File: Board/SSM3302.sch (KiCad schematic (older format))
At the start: 5 parts, among them U2 SSM3302ACPZ-R7

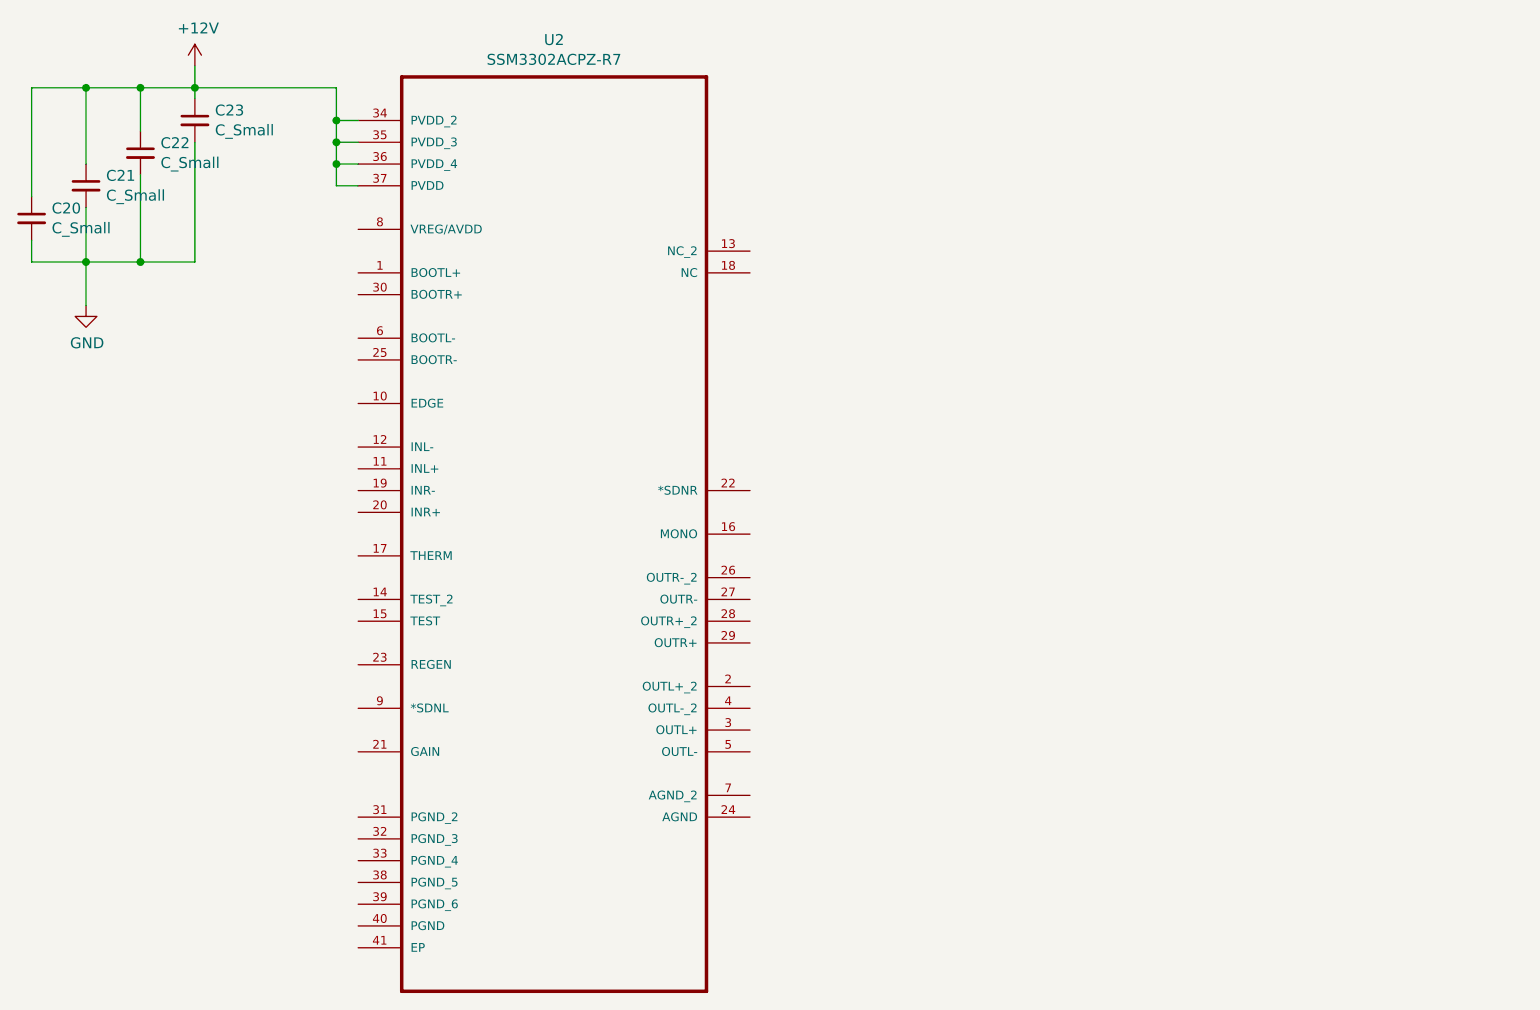
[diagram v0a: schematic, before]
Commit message: did some more stuff
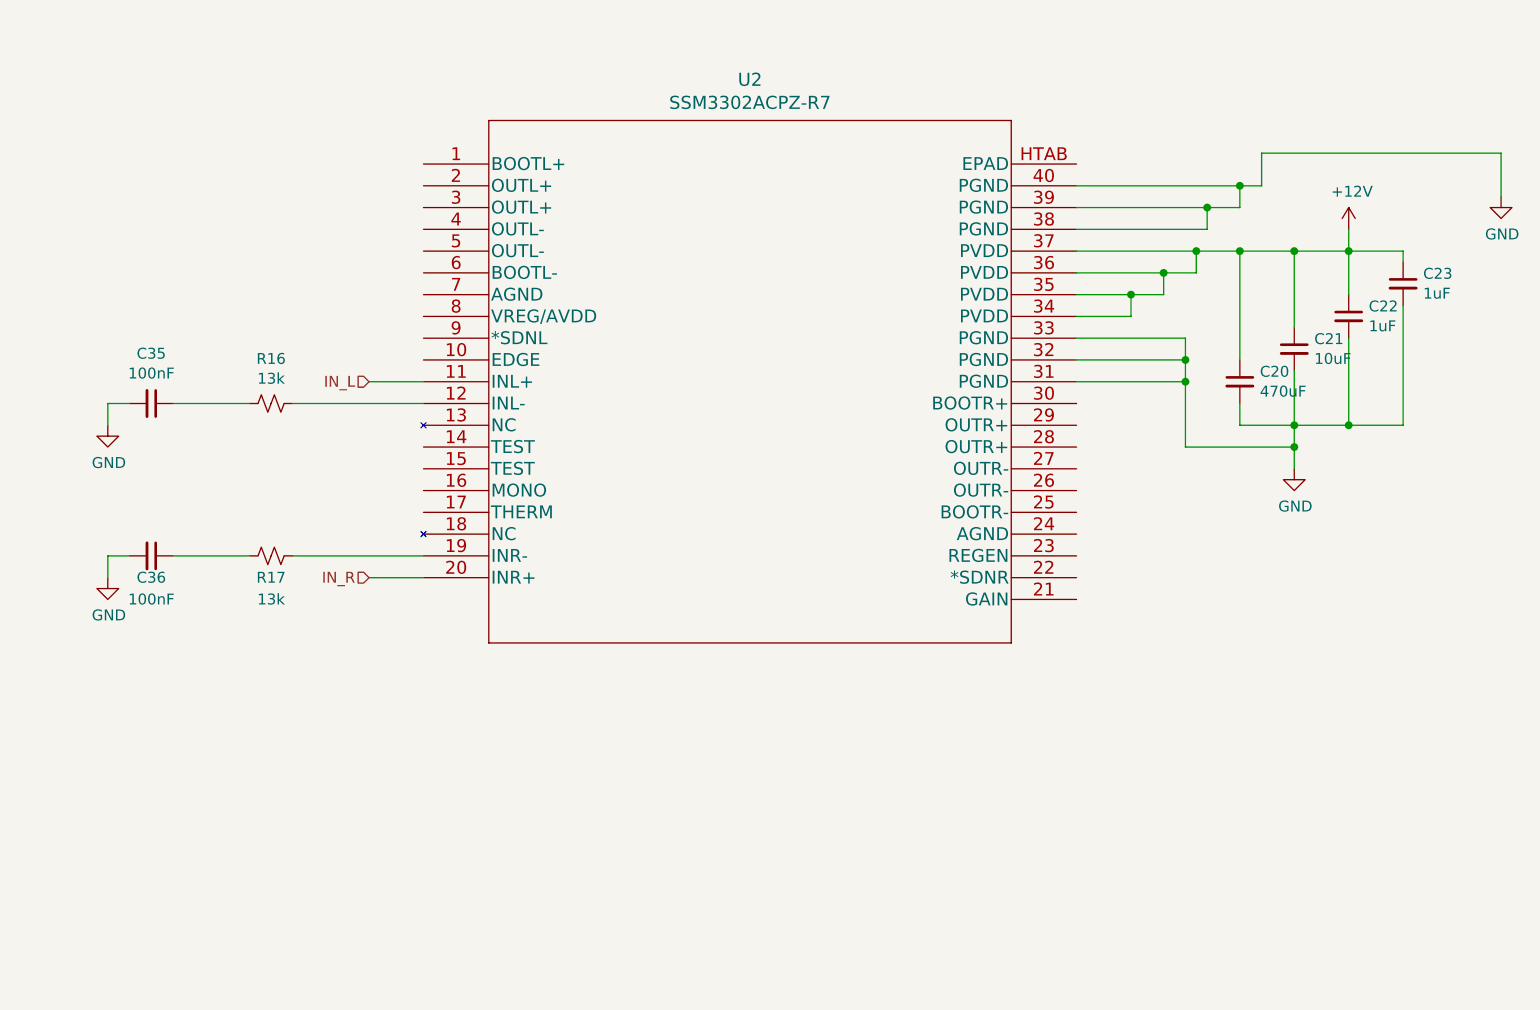
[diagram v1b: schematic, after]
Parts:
- removed U2: SSM3302ACPZ-R7, QFN50P600X600X80-41N, symbol SSM3302ACPZ-R7:SSM3302ACPZ-R7
- added C37, C38: 100nF, Capacitor_SMD:C_0805_2012Metric_Pad1.15x1.40mm_HandSolder, symbol Device:C_Small
- added R18, R19: 13k, Resistor_SMD:R_0805_2012Metric_Pad1.15x1.40mm_HandSolder, symbol Device:R_Small_US
- added U2: SSM3302ACPZ-R7, SSM3302:SSM3302ACPZ-R7, symbol 2019-11-17_04-12-08:SSM3302ACPZ-R7
- C20: value C_Small -> 470uF; footprint (none) -> Capacitor_SMD:C_0805_2012Metric_Pad1.15x1.40mm_HandSolder
- C21: value C_Small -> 10uF; footprint (none) -> Capacitor_SMD:C_0805_2012Metric_Pad1.15x1.40mm_HandSolder
- C22, C23: value C_Small -> 1uF; footprint (none) -> Capacitor_SMD:C_0805_2012Metric_Pad1.15x1.40mm_HandSolder
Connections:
- net +12V: now also U2.34 (PVDD), U2.35 (PVDD), U2.36 (PVDD), U2.37 (PVDD)
- net GND: now also C37.2, C38.2, U2.31 (PGND), U2.32 (PGND), U2.33 (PGND), U2.38 (PGND), U2.39 (PGND), U2.40 (PGND)
- new net: C37.1, R18.2
- new net: R18.1, U2.12 (INL-)
- new net: C38.1, R19.2
- new net: R19.1, U2.19 (INR-)
- new net IN_L: U2.11 (INL+)
- new net IN_R: U2.20 (INR+)
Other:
- moved on the sheet: C20, C21, C22, C23
